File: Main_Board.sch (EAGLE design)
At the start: 39 parts, among them U1 RN4020RN4020

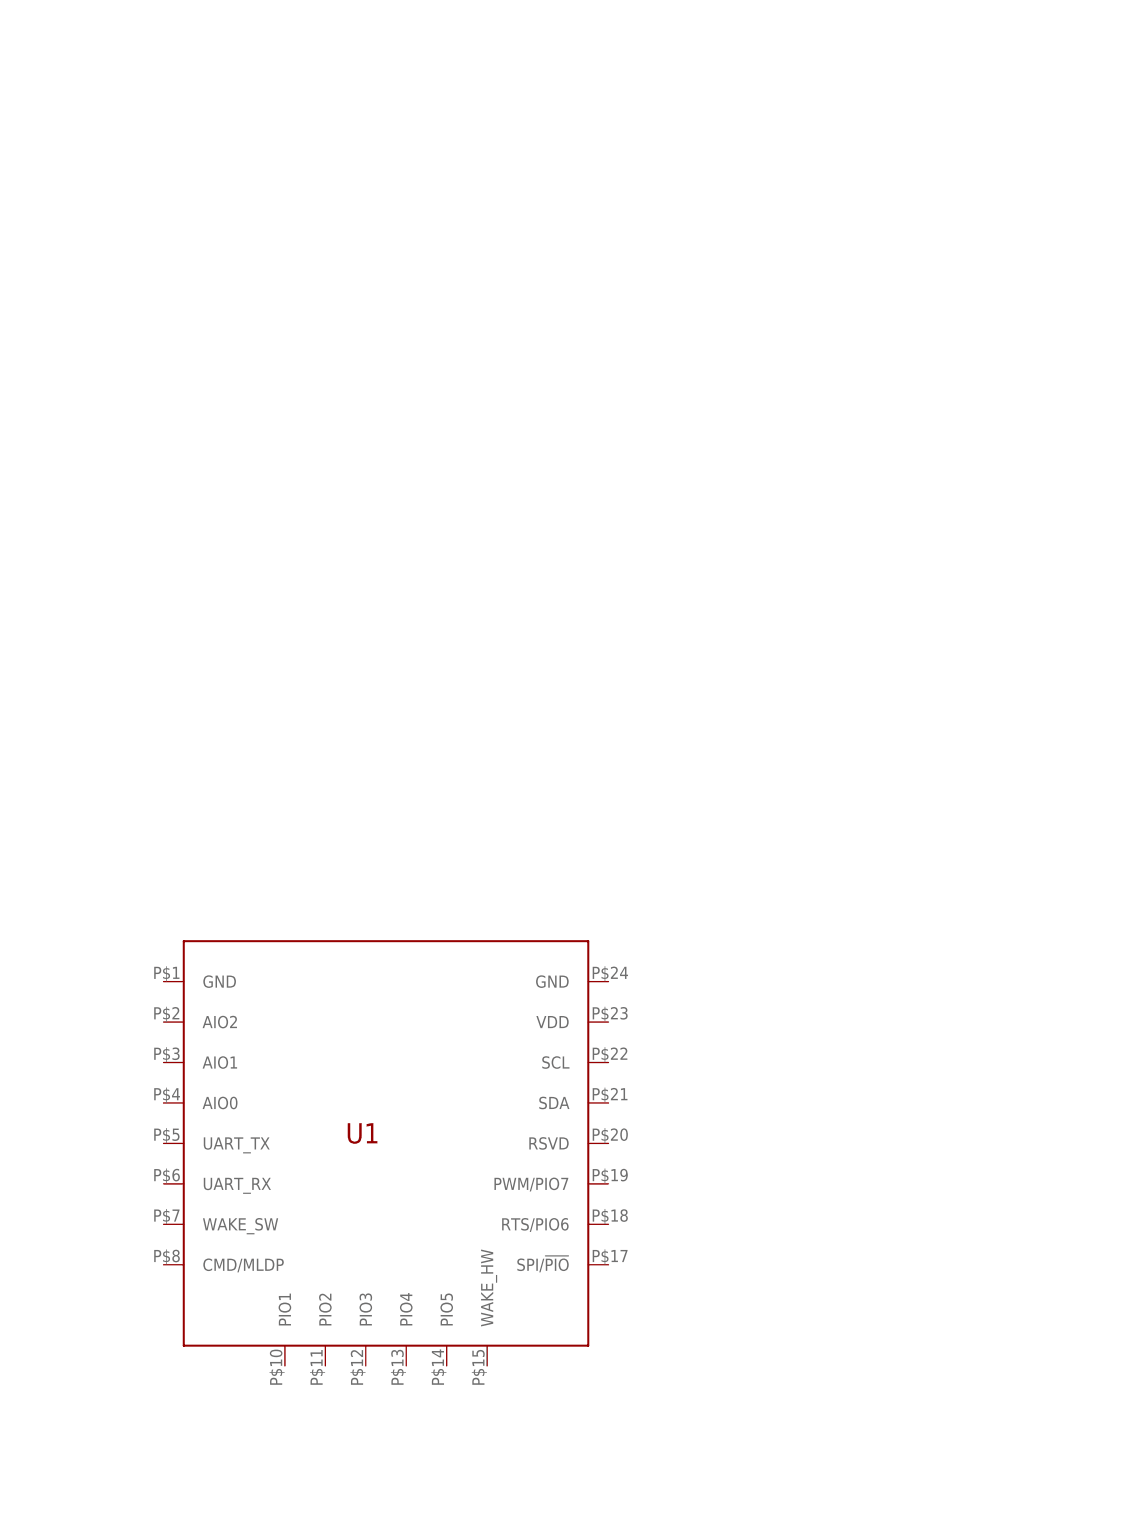
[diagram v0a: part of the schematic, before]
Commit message: Updates
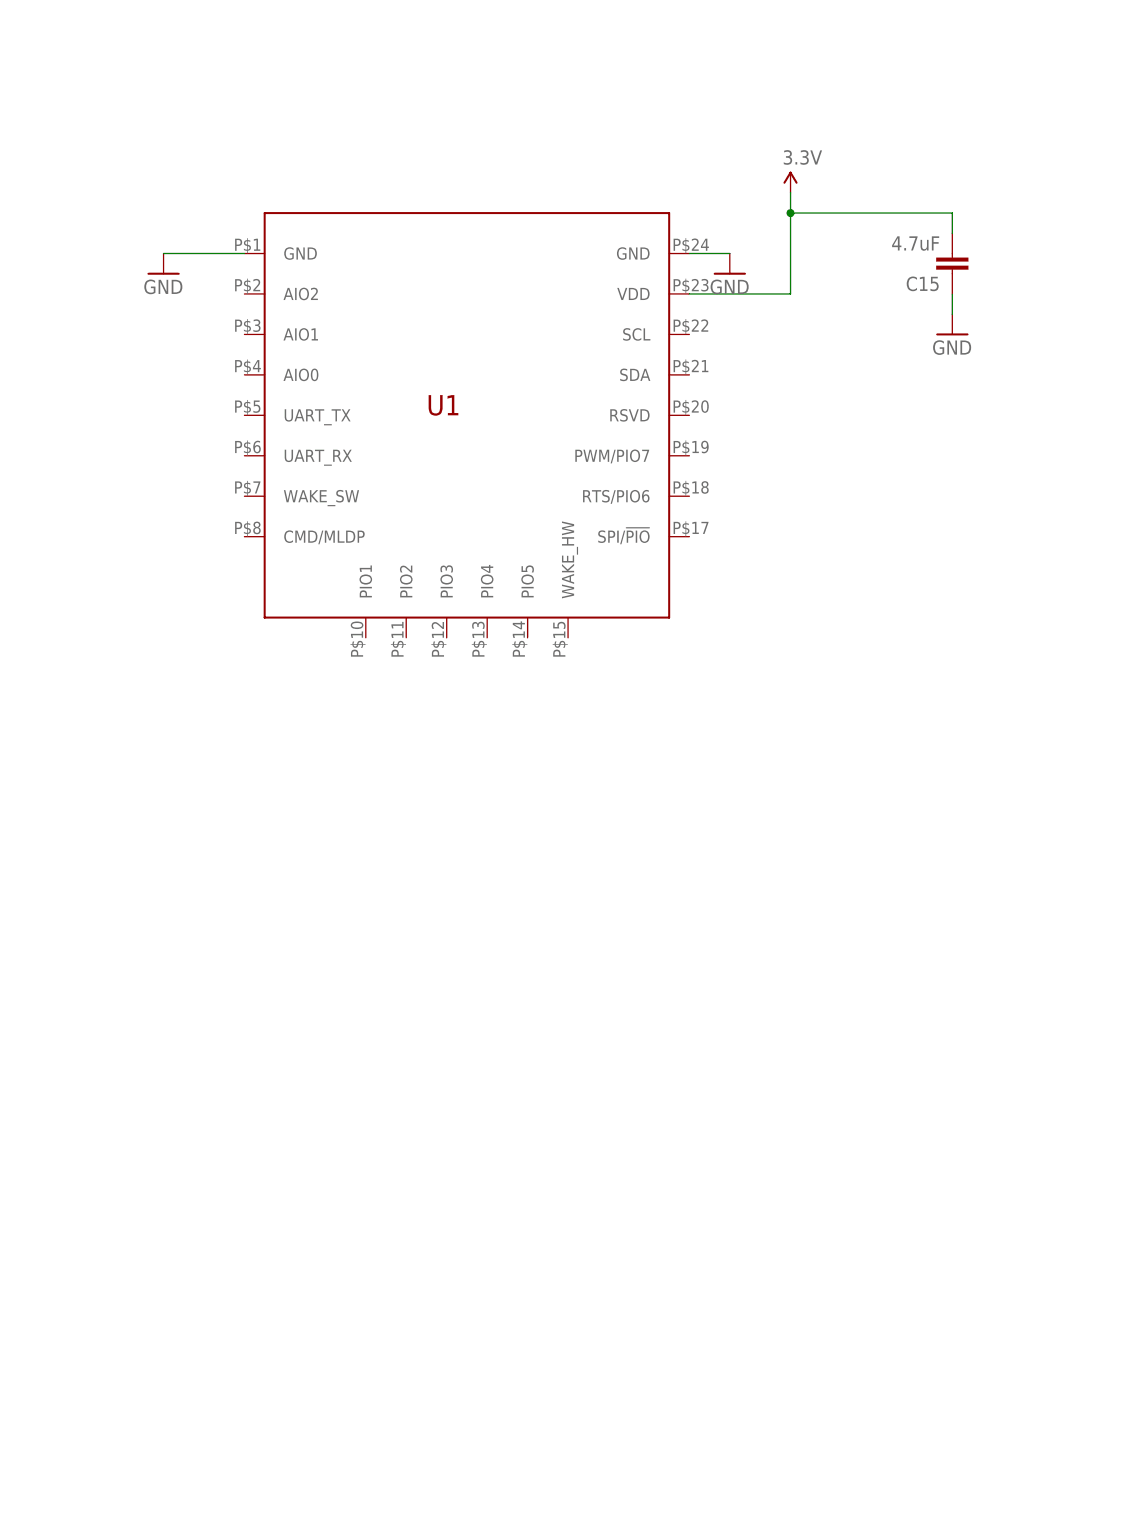
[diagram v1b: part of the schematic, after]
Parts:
- added C15: 4.7uF, SparkFun-Capacitors:CAP0805
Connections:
- net 3.3V: now also C15.2, U1.VDD
- net GND: now also C15.1, U1.GND@1, U1.GND@24
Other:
- moved on the sheet: U1
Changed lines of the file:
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@@
 <part name="SUPPLY16" library="SparkFun-Aesthetics" deviceset="5V" device=""/>
 <part name="SUPPLY17" library="SparkFun-Aesthetics" deviceset="5V" device=""/>
+<part name="SUPPLY18" library="SparkFun-Aesthetics" deviceset="3.3V" device=""/>
+<part name="C15" library="SparkFun-Capacitors" deviceset="CAP" device="0805" value="4.7uF"/>
+<part name="GND29" library="SparkFun-Aesthetics" deviceset="GND" device=""/>
+<part name="GND30" library="SparkFun-Aesthetics" deviceset="GND" device=""/>
+<part name="GND31" library="SparkFun-Aesthetics" deviceset="GND" device=""/>
 </parts>
 <sheets>
@@
 <instance part="U$6" gate="G$1" x="7.62" y="116.84"/>
 <instance part="U$7" gate="G$1" x="7.62" y="45.72"/>
-<instance part="U1" gate="G$1" x="495.3" y="-266.7"/>
+<instance part="U1" gate="G$1" x="505.46" y="-175.26"/>
 <instance part="SUPPLY5" gate="G$1" x="287.02" y="50.8"/>
 <instance part="SUPPLY6" gate="G$1" x="312.42" y="5.08"/>
@@
 <instance part="SUPPLY16" gate="G$1" x="193.04" y="50.8"/>
 <instance part="SUPPLY17" gate="G$1" x="193.04" y="35.56"/>
+<instance part="SUPPLY18" gate="G$1" x="546.1" y="-147.32"/>
+<instance part="C15" gate="G$1" x="566.42" y="-154.94" rot="R180"/>
+<instance part="GND29" gate="1" x="467.36" y="-157.48"/>
+<instance part="GND30" gate="1" x="538.48" y="-157.48"/>
+<instance part="GND31" gate="1" x="566.42" y="-165.1"/>
 </instances>
 <busses>
@@
 <wire x1="193.04" y1="30.48" x2="185.42" y2="30.48" width="0.1524" layer="91"/>
 </segment>
+<segment>
+<pinref part="U1" gate="G$1" pin="GND@24"/>
+<pinref part="GND30" gate="1" pin="GND"/>
+<wire x1="533.4" y1="-154.94" x2="538.48" y2="-154.94" width="0.1524" layer="91"/>
+</segment>
+<segment>
+<pinref part="C15" gate="G$1" pin="1"/>
+<pinref part="GND31" gate="1" pin="GND"/>
+<wire x1="566.42" y1="-162.56" x2="566.42" y2="-160.02" width="0.1524" layer="91"/>
+</segment>
+<segment>
+<pinref part="U1" gate="G$1" pin="GND@1"/>
+<pinref part="GND29" gate="1" pin="GND"/>
+<wire x1="477.52" y1="-154.94" x2="467.36" y2="-154.94" width="0.1524" layer="91"/>
+</segment>
 </net>
 <net name="N$1" class="0">
@@
 <wire x1="193.04" y1="129.54" x2="193.04" y2="132.08" width="0.1524" layer="91"/>
 </segment>
-</net>
+<segment>
+<pinref part="U1" gate="G$1" pin="VDD"/>
+<wire x1="533.4" y1="-160.02" x2="546.1" y2="-160.02" width="0.1524" layer="91"/>
+<pinref part="SUPPLY18" gate="G$1" pin="3.3V"/>
+<wire x1="546.1" y1="-160.02" x2="546.1" y2="-149.86" width="0.1524" layer="91"/>
+<pinref part="C15" gate="G$1" pin="2"/>
+<wire x1="546.1" y1="-149.86" x2="546.1" y2="-147.32" width="0.1524" layer="91"/>
+<wire x1="566.42" y1="-152.4" x2="566.42" y2="-149.86" width="0.1524" layer="91"/>
+<wire x1="566.42" y1="-149.86" x2="546.1" y2="-149.86" width="0.1524" layer="91"/>
+<junction x="546.1" y="-149.86"/>
+</segment>
+</net>
